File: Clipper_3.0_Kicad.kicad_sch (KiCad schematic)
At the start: 25 parts, among them J1 Conn_01x08_Pin, J10 Conn_01x19_Socket, J11 Screw_Terminal_01x02, J12 Conn_01x01_Socket, J13 Conn_01x01_Socket, J14 Conn_01x01_Socket, J15 Conn_01x01_Socket, J16 Conn_01x01_Pin, J17 Conn_01x01_Pin, J18 Conn_01x01_Pin, J19 Conn_01x01_Pin, J2 Conn_01x08_Pin, J3 Conn_01x08_Pin, J4 Conn_01x08_Socket, J5 Conn_01x08_Socket, J6 Conn_01x08_Socket, J7 Conn_01x19_Pin, J8 Conn_01x19_Pin, J9 Conn_01x19_Socket, M1 Motor_Derecho, M2 Motor_Îzquierdo, U1 ESP32-DevKitC, U2 TB6612FNG_MODULE, U3 GY-521 MODULE, U4 DC/DC MINI-360

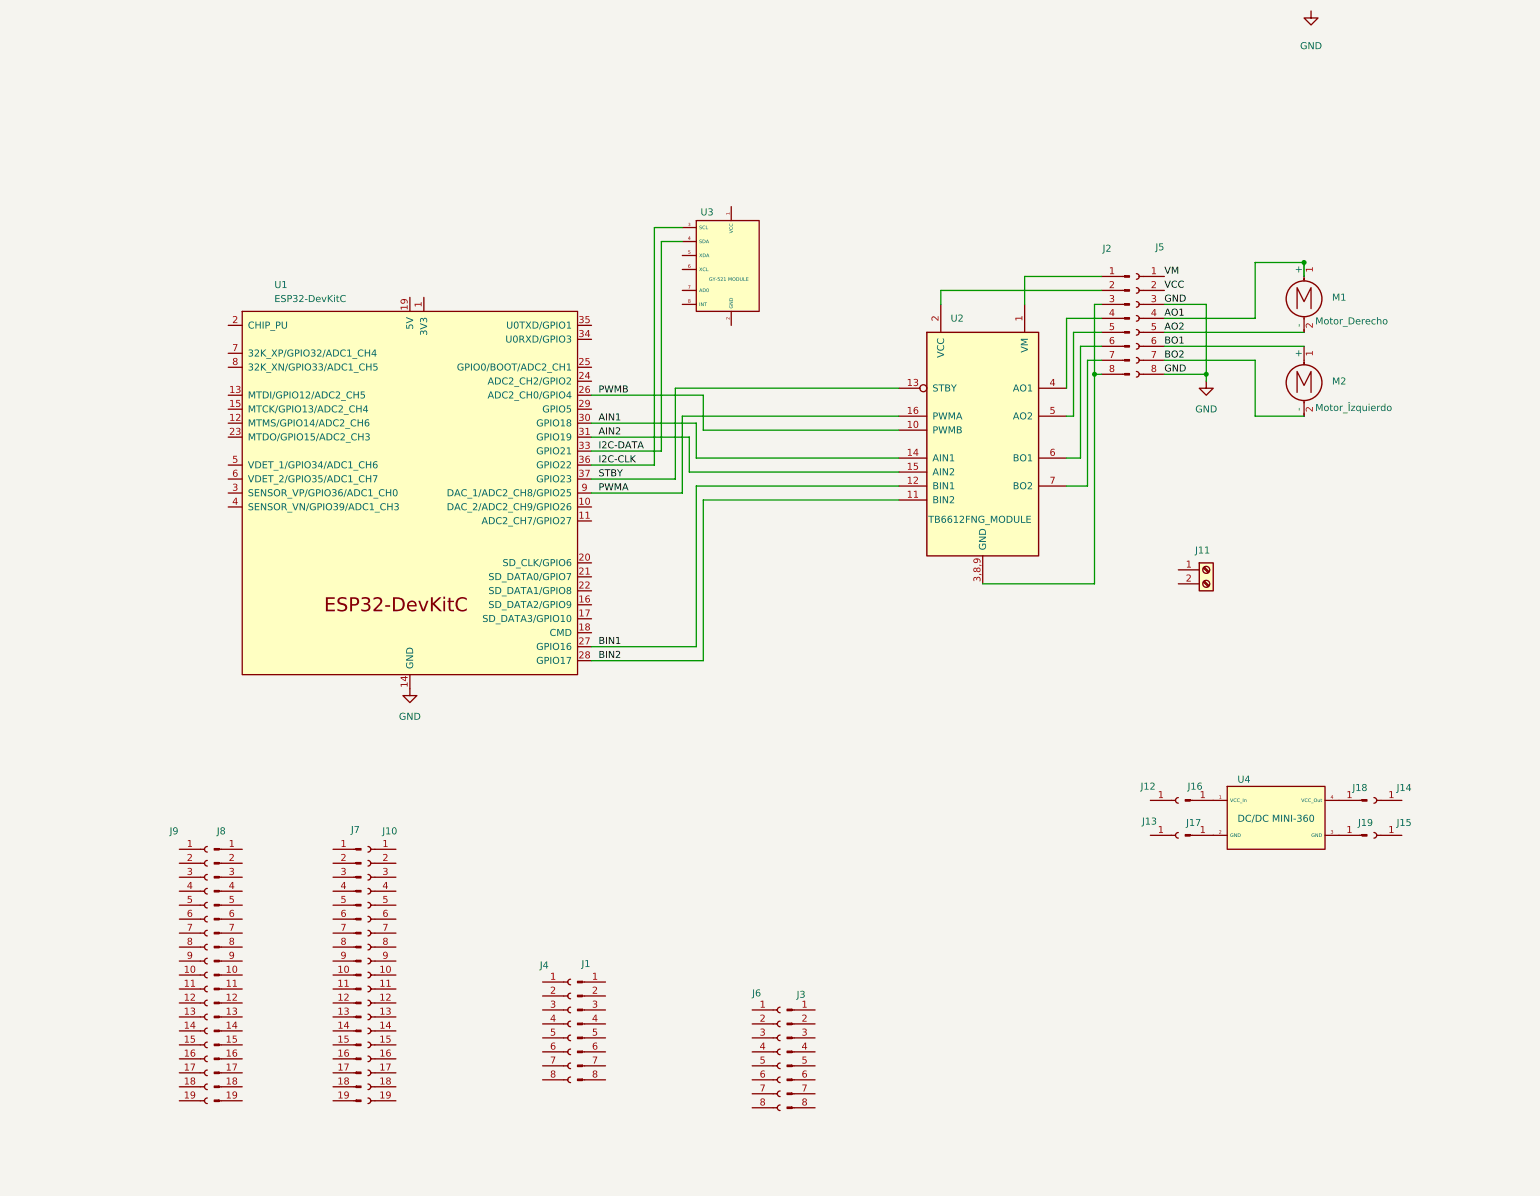
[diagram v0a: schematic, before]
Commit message: Actualizacion de avance en SCH
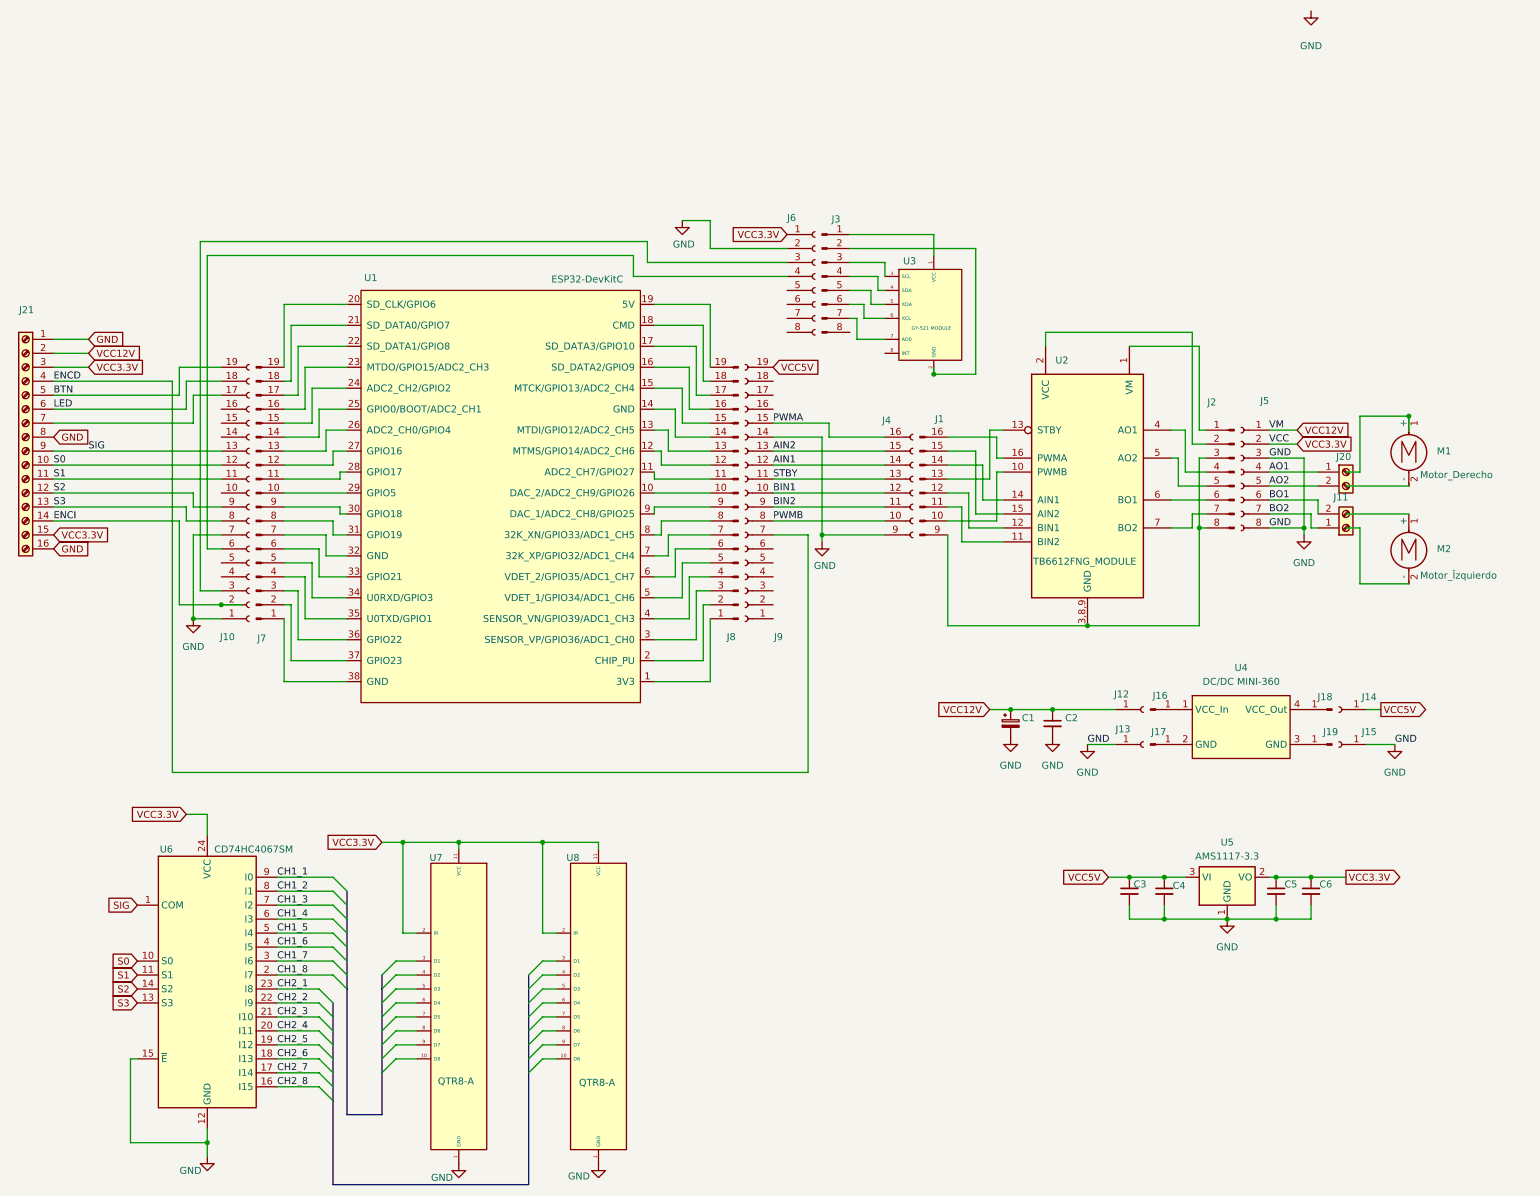
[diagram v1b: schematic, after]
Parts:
- removed U1: ESP32-DevKitC, Espressif:ESP32-DevKitC, symbol PCM_Espressif:ESP32-DevKitC
- added C1: C_Polarized_Small, Capacitor_THT:CP_Radial_D8.0mm_P3.50mm, symbol Device:C_Polarized_Small
- added C2, C3, C4, C5, C6: C_Small, symbol Device:C_Small
- added J20: Screw_Terminal_01x02, TerminalBlock:TerminalBlock_Xinya_XY308-2.54-2P_1x02_P2.54mm_Horizontal, symbol Connector:Screw_Terminal_01x02
- added J21: Screw_Terminal_01x16, TerminalBlock:TerminalBlock_Xinya_XY308-2.54-16P_1x16_P2.54mm_Horizontal, symbol Connector:Screw_Terminal_01x16
- added U1: ESP32-DevKitC, Espressif:ESP32-DevKitC, symbol Personal:ESP32-DevKitC
- added U5: AMS1117-3.3, Package_TO_SOT_SMD:SOT-223-3_TabPin2, symbol Regulator_Linear:AMS1117-3.3
- added U6: CD74HC4067SM, Package_SO:SSOP-24_5.3x8.2mm_P0.65mm, symbol 74xx:CD74HC4067SM
- added U7, U8: QTR8-A, symbol Personal:QTR8-A
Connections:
- net I2C-CLK is gone; now on an unnamed net: U3.3 (SCL)
- net I2C-DATA is gone; now on an unnamed net: U3.4 (SDA)
- net VCC is gone; now on net VCC3.3V: J5.2 (Pin_2)
- net VM is gone; now on net VCC12V: J5.1 (Pin_1)
- net AIN1: now also J4.14 (Pin_3), J9.12 (Pin_12); no longer U2.14 (AIN1)
- net AIN2: now also J4.15 (Pin_2), J9.13 (Pin_13); no longer U2.15 (AIN2)
- net AO1: now also J20.1 (Pin_1); no longer M1.1 (+)
- net AO2: now also J20.2 (Pin_2); no longer M1.2 (-)
- net BIN1: now also J4.12 (Pin_5), J9.10 (Pin_10); no longer U2.12 (BIN1)
- net BIN2: now also J4.11 (Pin_6), J9.9 (Pin_9); no longer U2.11 (BIN2)
- net BO1: now also J11.2 (Pin_2); no longer M2.1 (+)
- net BO2: now also J11.1 (Pin_1); no longer M2.2 (-)
- net GND: now also J10.1 (Pin_1), J10.7 (Pin_7), J13.1 (Pin_1), J15.1 (Pin_1), J4.9 (Pin_8), J6.2 (Pin_2), J9.14 (Pin_14), C1.2, C2.2, C3.2, C4.2, C5.2, C6.2, J21.1 (Pin_1), J21.16 (Pin_16), J21.8 (Pin_8), U5.1 (GND), U6.12 (GND), U6.15 (~{E}), U7.1 (GND), U8.1 (GND)
- net PWMA: now also J4.16 (Pin_1), J9.15 (Pin_15); no longer U2.16 (PWMA)
- net PWMB: now also J4.10 (Pin_7), J9.8 (Pin_8); no longer U2.10 (PWMB)
- net STBY: now also J4.13 (Pin_4), J9.11 (Pin_11); no longer U2.13 (STBY)
- net at J3.1 (Pin_1): now also U3.1 (VCC)
- net at J3.2 (Pin_2): now also U3.2 (GND)
- net at J3.5 (Pin_5): now also U3.5 (XDA)
- net at J3.6 (Pin_6): now also U3.6 (XCL)
- net at J3.7 (Pin_7): now also U3.7 (AD0)
- net at J2.3 (Pin_3), J2.8 (Pin_8), U2.3,8,9 (GND): now also J1.9 (Pin_8)
- net at J7.1 (Pin_1): now also U1.38 (GND)
- net at J7.10 (Pin_10): now also U1.29 (GPIO5)
- net at J7.11 (Pin_11): now also U1.28 (GPIO17)
- net at J7.12 (Pin_12): now also U1.27 (GPIO16)
- net at J7.13 (Pin_13): now also U1.26 (ADC2_CH0/GPIO4)
- net at J7.14 (Pin_14): now also U1.25 (GPIO0/BOOT/ADC2_CH1)
- net at J7.15 (Pin_15): now also U1.24 (ADC2_CH2/GPIO2)
- net at J7.16 (Pin_16): now also U1.23 (MTDO/GPIO15/ADC2_CH3)
- net at J7.17 (Pin_17): now also U1.22 (SD_DATA1/GPIO8)
- net at J7.18 (Pin_18): now also U1.21 (SD_DATA0/GPIO7)
- net at J7.19 (Pin_19): now also U1.20 (SD_CLK/GPIO6)
- net at J7.2 (Pin_2): now also U1.37 (GPIO23)
- net at J7.3 (Pin_3): now also U1.36 (GPIO22)
- net at J7.4 (Pin_4): now also U1.35 (U0TXD/GPIO1)
- net at J7.5 (Pin_5): now also U1.34 (U0RXD/GPIO3)
- net at J7.6 (Pin_6): now also U1.33 (GPIO21)
- net at J7.7 (Pin_7): now also U1.32 (GND)
- net at J7.8 (Pin_8): now also U1.31 (GPIO19)
- net at J7.9 (Pin_9): now also U1.30 (GPIO18)
- net S1: now reaches J10.11 (Pin_11)
- net S1: now also J21.11 (Pin_11), U6.11 (S1)
- net S0: now reaches J10.12 (Pin_12)
- net S0: now also J21.10 (Pin_10), U6.10 (S0)
- net SIG: now reaches J10.13 (Pin_13)
- net SIG: now also J21.9 (Pin_9), U6.1 (COM)
- net at J10.17 (Pin_17): now also J21.7 (Pin_7)
- net LED: now reaches J10.18 (Pin_18)
- net LED: now also J21.6 (Pin_6)
- net BTN: now reaches J10.19 (Pin_19)
- net BTN: now also J21.5 (Pin_5)
- net ENCI: now reaches J10.2 (Pin_2)
- net ENCI: now also J21.14 (Pin_14)
- net at J10.3 (Pin_3): now also J6.3 (Pin_3)
- net at J10.6 (Pin_6): now also J6.4 (Pin_4)
- net S3: now reaches J10.8 (Pin_8)
- net S3: now also J21.13 (Pin_13), U6.13 (S3)
- net S2: now reaches J10.9 (Pin_9)
- net S2: now also J21.12 (Pin_12), U6.14 (S2)
- net VCC3.3V: now reaches J6.1 (Pin_1)
- net VCC3.3V: now also C5.1, C6.1, J21.15 (Pin_15), J21.3 (Pin_3), U5.2 (VO), U6.24 (VCC), U7.11 (VCC), U7.2 (IR), U8.11 (VCC), U8.2 (IR)
- net VCC5V: now reaches J9.19 (Pin_19)
- net VCC5V: now also J14.1 (Pin_1), C3.1, C4.1, U5.3 (VI)
- net ENCD: now reaches J9.7 (Pin_7)
- net ENCD: now also J21.4 (Pin_4)
- net VCC12V: now reaches J12.1 (Pin_1)
- net VCC12V: now also C1.1, C2.1, J21.2 (Pin_2)
- net at J8.1 (Pin_1): now also U1.1 (3V3)
- net at J8.10 (Pin_10): now also U1.10 (DAC_2/ADC2_CH9/GPIO26)
- net at J8.11 (Pin_11): now also U1.11 (ADC2_CH7/GPIO27)
- net at J8.12 (Pin_12): now also U1.12 (MTMS/GPIO14/ADC2_CH6)
- net at J8.13 (Pin_13): now also U1.13 (MTDI/GPIO12/ADC2_CH5)
- net at J8.14 (Pin_14): now also U1.14 (GND)
- net at J8.15 (Pin_15): now also U1.15 (MTCK/GPIO13/ADC2_CH4)
- net at J8.16 (Pin_16): now also U1.16 (SD_DATA2/GPIO9)
- net at J8.17 (Pin_17): now also U1.17 (SD_DATA3/GPIO10)
- net at J8.18 (Pin_18): now also U1.18 (CMD)
- net at J8.19 (Pin_19): now also U1.19 (5V)
- net at J8.2 (Pin_2): now also U1.2 (CHIP_PU)
- net at J8.3 (Pin_3): now also U1.3 (SENSOR_VP/GPIO36/ADC1_CH0)
- net at J8.4 (Pin_4): now also U1.4 (SENSOR_VN/GPIO39/ADC1_CH3)
- net at J8.5 (Pin_5): now also U1.5 (VDET_1/GPIO34/ADC1_CH6)
- net at J8.6 (Pin_6): now also U1.6 (VDET_2/GPIO35/ADC1_CH7)
- net at J8.7 (Pin_7): now also U1.7 (32K_XP/GPIO32/ADC1_CH4)
- net at J8.8 (Pin_8): now also U1.8 (32K_XN/GPIO33/ADC1_CH5)
- net at J8.9 (Pin_9): now also U1.9 (DAC_1/ADC2_CH8/GPIO25)
- new net: J1.10 (Pin_7), U2.10 (PWMB)
- new net: J1.11 (Pin_6), U2.11 (BIN2)
- new net: J1.12 (Pin_5), U2.12 (BIN1)
- new net: J1.13 (Pin_4), U2.13 (STBY)
- new net: J1.14 (Pin_3), U2.14 (AIN1)
- new net: J1.15 (Pin_2), U2.15 (AIN2)
- new net: J1.16 (Pin_1), U2.16 (PWMA)
- new net CH1_1: U6.9 (I0)
- new net CH1_2: U6.8 (I1)
- new net CH1_3: U6.7 (I2)
- new net CH1_4: U6.6 (I3)
- new net CH1_5: U6.5 (I4)
- new net CH1_6: U6.4 (I5)
- new net CH1_7: U6.3 (I6)
- new net CH1_8: U6.2 (I7)
- new net CH2_1: U6.23 (I8)
- new net CH2_2: U6.22 (I9)
- new net CH2_3: U6.21 (I10)
- new net CH2_4: U6.20 (I11)
- new net CH2_5: U6.19 (I12)
- new net CH2_6: U6.18 (I13)
- new net CH2_7: U6.17 (I14)
- new net CH2_8: U6.16 (I15)
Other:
- moved on the sheet: J10, J11, J12, J13, J14, J15, J16, J17, J18, J19, J2, J3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
